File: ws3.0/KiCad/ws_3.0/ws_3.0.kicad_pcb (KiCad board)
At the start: 2 copper layers, 72.8 x 113.9 mm, 55 parts, among them J1 ISP TINY, J2 Rain, J3 Wind, J4 Temp, J5 2604-1102, J6 ISP MEGA, J7 FTDI MEGA, SW1 SW_DIP_x03, SW2 RESET TINY, SW3 RESET ATMEGA, U1 ATmega328P-A, U2 LF33_TO220, U3 ATtiny85V-10S, U4 XC6206PxxxMR, U5 RFM95W-868S2, Y1 Crystal

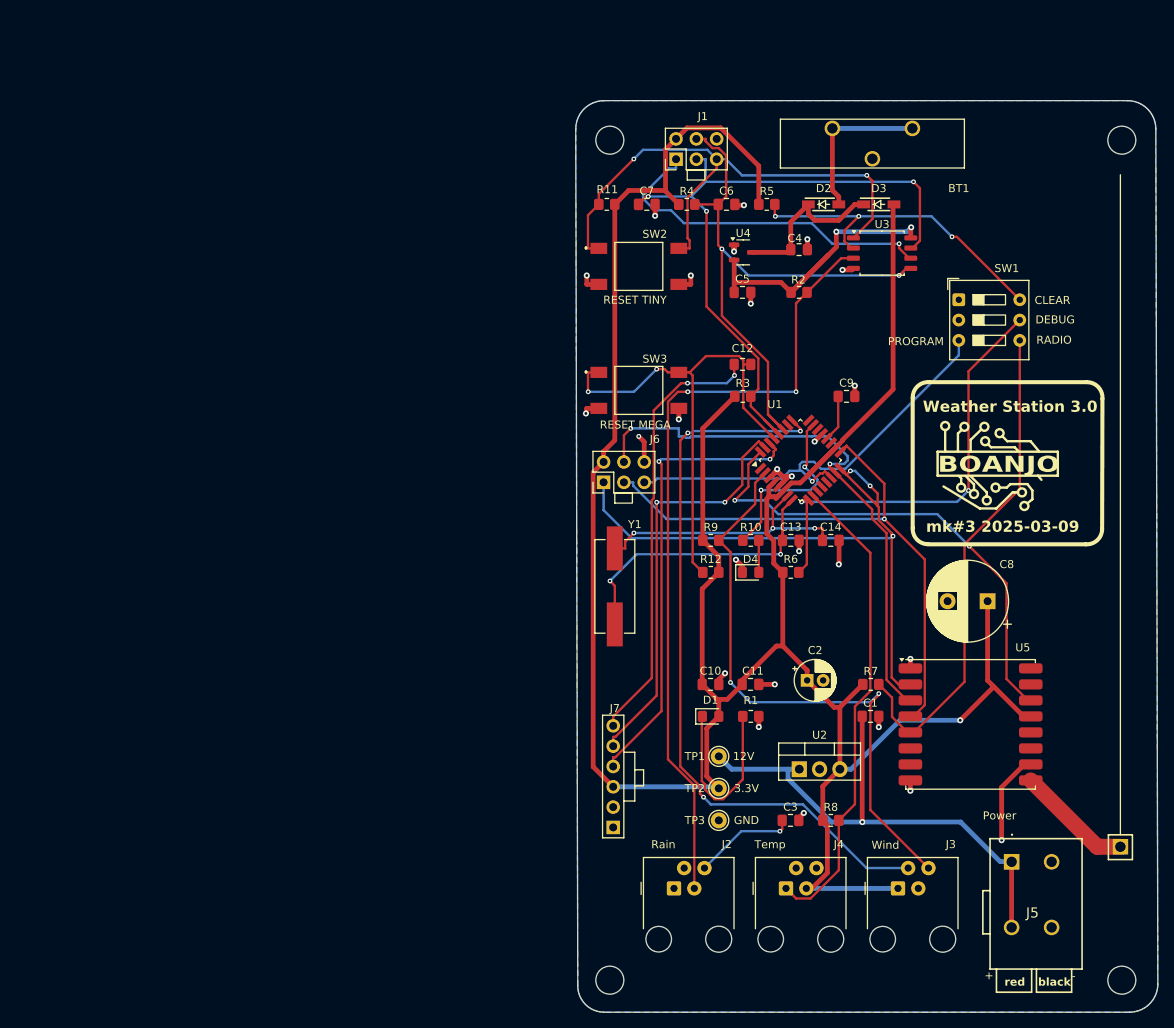
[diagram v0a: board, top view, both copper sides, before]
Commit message: Updates for mk #5
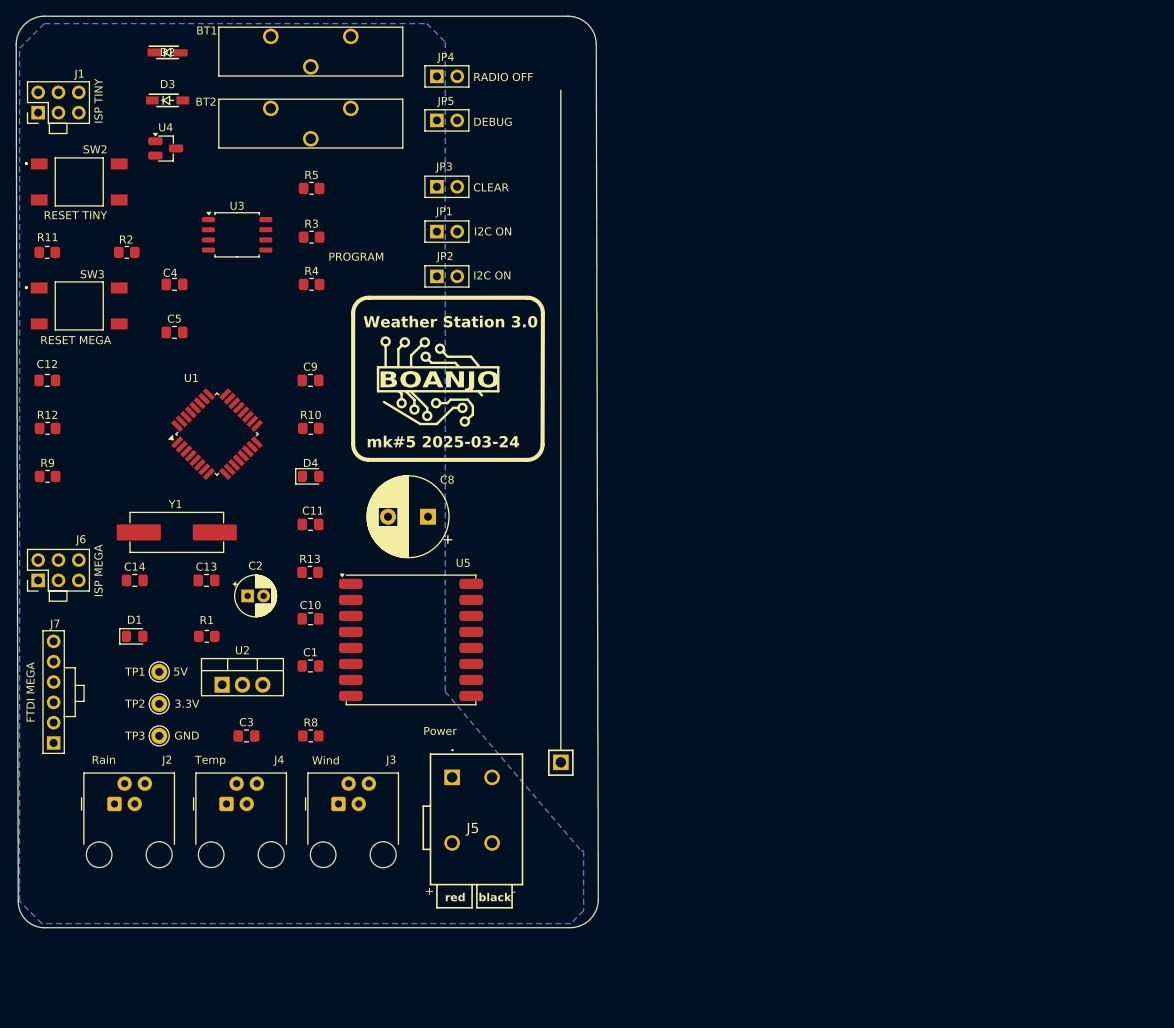
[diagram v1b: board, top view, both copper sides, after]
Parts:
- removed C6, C7: 0.1uF, Capacitor_SMD:C_0805_2012Metric_Pad1.18x1.45mm_HandSolder
- removed R6, R7: 4k7, Resistor_SMD:R_0805_2012Metric_Pad1.20x1.40mm_HandSolder
- removed SW1: SW_DIP_x03, Button_Switch_THT:SW_DIP_SPSTx03_Slide_9.78x9.8mm_W7.62mm_P2.54mm
- removed UNK_HOLE_0: , dummyfp0
- removed UNK_HOLE_1: , dummyfp1
- removed UNK_HOLE_2: , dummyfp2
- removed UNK_HOLE_3: , dummyfp3
- added BT2: CR2032, boan_devices:CR2032 standing 1074, F.Cu at (74.0, 49.0)
- added JP1: SCL, boan_devices:Jumper 2p, F.Cu at (96.1, 64.4)
- added JP2: SDA, boan_devices:Jumper 2p, F.Cu at (96.1, 70.0)
- added JP3: CLEAR, boan_devices:Jumper 2p, F.Cu at (96.1, 58.8)
- added JP4: PROGRAM MEGA, boan_devices:Jumper 2p, F.Cu at (96.1, 45.0)
- added JP5: DEBUG, boan_devices:Jumper 2p, F.Cu at (96.1, 50.5)
- added R13: 4k7, Resistor_SMD:R_0805_2012Metric_Pad1.20x1.40mm_HandSolder, F.Cu at (78.9, 107.0)
- D2: value 1N5819WS -> BAP70; footprint boan_devices:1N5819HW -> boan_devices:BAP70
- R1: value 330 -> 1k
- U4: footprint Package_TO_SOT_SMD:SOT-23-3 -> boan_devices:SOT-23
- moved D3 89.8 mm to (61.1, 48.0)
- moved C14 87.1 mm to (57.0, 108.0)
- moved C12 86.9 mm to (46.1, 83.0)
- moved R12 84.8 mm to (46.1, 89.0)
- moved R2 84.2 mm to (56.0, 67.0)
- moved D2 84.2 mm to (61.1, 42.0)
- moved R9 83.3 mm to (46.1, 95.0)
- moved U3 80.7 mm to (69.8, 64.8)
- moved J1 79.9 mm to (44.9, 49.5)
- moved C4 78.2 mm to (62.0, 71.0)
- moved U4 73.3 mm to (60.9, 54.0)
- moved C13 73.2 mm to (66.0, 108.0)
- moved U1 73.0 mm to (67.3, 89.7)
- moved U2 72.9 mm to (67.9, 121.0)
- moved D1 72.7 mm to (57.0, 115.0)
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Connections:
- BT1 pad 2: GND -> BAT
- C1 pad 1: /power/RAW -> RAW
- C12 pad 1: Net-(U1-~{RESET}/PC6) -> Net-(J6-~{RST})
- D3 pad 2: +3.3V -> RAW
- J1 pad 2: +3.3V -> RAW
- J1 pad 3: I2C_SCL -> Net-(J1-SCK)
- J1 pad 4: I2C_SDA -> Net-(J1-MOSI)
- J5 pad 1: /power/RAW -> RAW
- J5 pad 2: /power/RAW -> RAW
- J6 pad 2: +3.3V -> RAW
- J6 pad 5: SS -> Net-(J6-~{RST})
- R11 pad 2: +3.3V -> BACKUP_POWER
- R12 pad 1: Net-(U1-~{RESET}/PC6) -> Net-(J6-~{RST})
- R5 pad 1: +3.3V -> BACKUP_POWER
- SW3 pad 1: Net-(U1-~{RESET}/PC6) -> Net-(J6-~{RST})
- SW3 pad 3: Net-(U1-~{RESET}/PC6) -> Net-(J6-~{RST})
- TP1 pad 1: /power/RAW -> RAW
- U1 pad 14: SS -> NSS
- U1 pad 29: Net-(U1-~{RESET}/PC6) -> Net-(J6-~{RST})
- U2 pad 1: /power/RAW -> RAW
- U3 pad 5: I2C_SDA -> Net-(J1-MOSI)
- U3 pad 7: I2C_SCL -> Net-(J1-SCK)
- U5 pad 5: OPT_PROGRAM -> NSS
- U5 pad 6: unconnected-(U5-RESET-Pad6) -> Net-(U5-RESET)
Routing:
- net +3.3V: track 353.4 -> 0.00 mm, vias 1 -> 0
- net RAIN: track 99.3 -> 0.00 mm, vias 2 -> 0
- net WIND_DIR: track 93.0 -> 0.00 mm, vias 3 -> 0
- net I2C_SCL: track 86.9 -> 0.00 mm, vias 3 -> 0
- net MISO: track 80.8 -> 0.00 mm, vias 3 -> 0
- net SCK: track 75.7 -> 0.00 mm, vias 1 -> 0
- net WIND_SPEED: track 75.0 -> 0.00 mm, vias 2 -> 0
- net I2C_SDA: track 73.7 -> 0.00 mm, vias 2 -> 0
- net MOSI: track 71.9 -> 0.00 mm, vias 2 -> 0
- net Net-(J1-~{RST}): track 69.0 -> 0.00 mm, vias 2 -> 0
- net /power/RAW: track 65.6 -> 0.00 mm, vias 1 -> 0
- net Net-(U1-~{RESET}/PC6): track 63.6 -> 0.00 mm, vias 2 -> 0
- net OPT_PROGRAM: track 62.8 -> 0.00 mm
- net DIO0: track 61.7 -> 0.00 mm, vias 2 -> 0
- net GND: track 61.3 -> 0.00 mm, vias 26 -> 0
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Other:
- board text added: "5V"
- board text added: "FTDI MEGA"
- board text added: "I2C ON"
- board text added: "RADIO OFF"
- board text added: "mk#5 2025-03-24"
- board text removed: "12V"
- board text removed: "RADIO"
- board text removed: "mk#3 2025-03-09"

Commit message: PCBWAYs delivery 2025-04-16 mk#5 of ws3.0
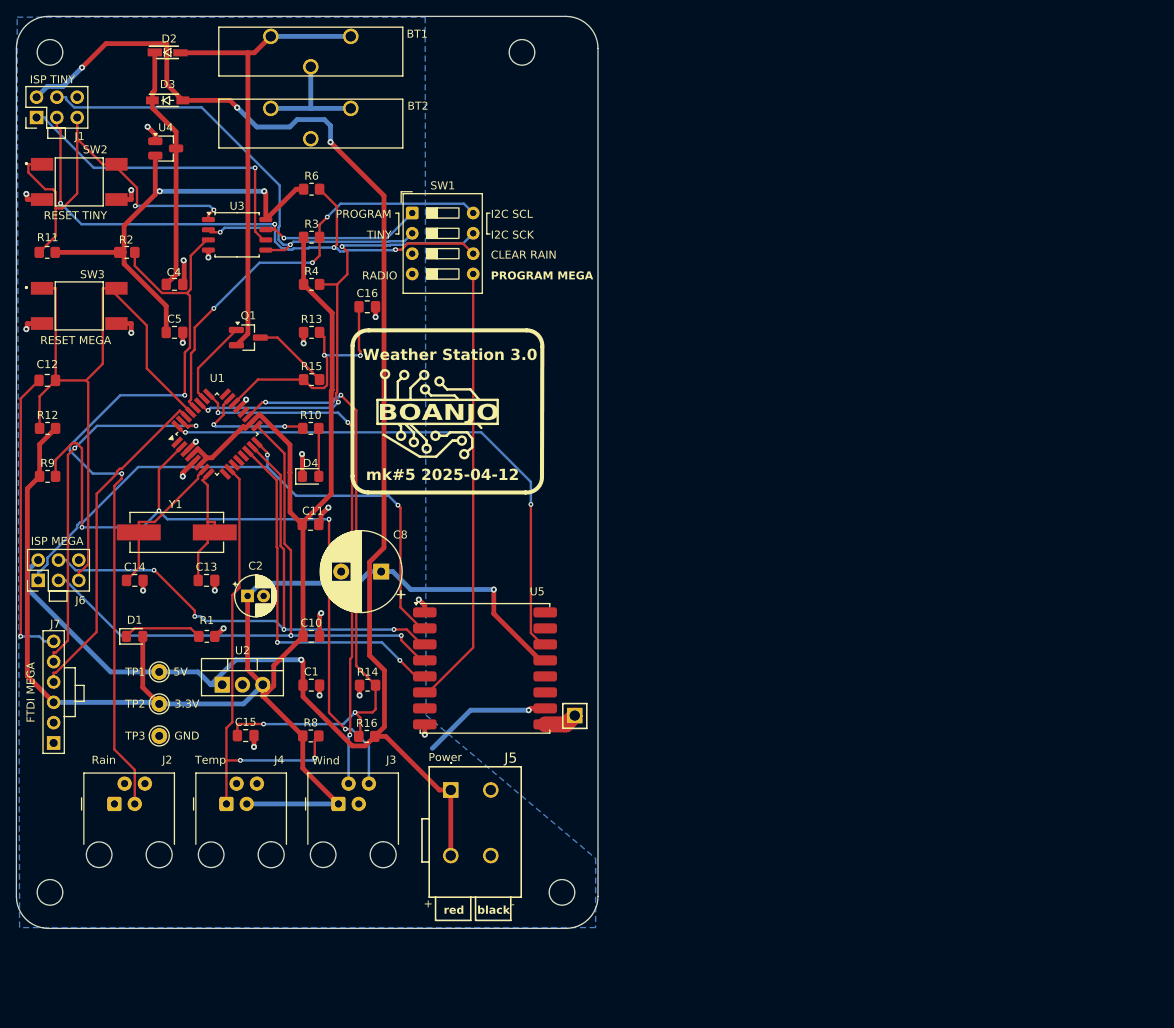
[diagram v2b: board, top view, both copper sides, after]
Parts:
- removed C3, C9: 0.1uF, Capacitor_SMD:C_0805_2012Metric_Pad1.18x1.45mm_HandSolder
- removed JP1: SCL, boan_devices:Jumper 2p
- removed JP2: SDA, boan_devices:Jumper 2p
- removed JP3: CLEAR, boan_devices:Jumper 2p
- removed JP4: PROGRAM MEGA, boan_devices:Jumper 2p
- removed JP5: DEBUG, boan_devices:Jumper 2p
- removed R5: 4k7, Resistor_SMD:R_0805_2012Metric_Pad1.20x1.40mm_HandSolder
- added C15: 0.1uF, Capacitor_SMD:C_0805_2012Metric_Pad1.18x1.45mm_HandSolder, F.Cu at (70.9, 127.4)
- added C16: 0.1uF, Capacitor_SMD:C_0805_2012Metric_Pad1.18x1.45mm_HandSolder, F.Cu at (86.1, 73.8)
- added MH1: MountingHole_3.2mm_M3, MountingHole:MountingHole_3.2mm_M3, F.Cu at (46.4, 42.0)
- added MH2: MountingHole_3.2mm_M3, MountingHole:MountingHole_3.2mm_M3, F.Cu at (105.4, 42.0)
- added MH3: MountingHole_3.2mm_M3, MountingHole:MountingHole_3.2mm_M3, F.Cu at (46.4, 147.0)
- added MH4: MountingHole_3.2mm_M3, MountingHole:MountingHole_3.2mm_M3, F.Cu at (110.4, 147.0)
- added Q1: ISS55EP06LMXTSA1, Package_TO_SOT_SMD:SOT-23_Handsoldering, F.Cu at (71.2, 77.7)
- added R14: 100k, Resistor_SMD:R_0805_2012Metric_Pad1.20x1.40mm_HandSolder, F.Cu at (86.1, 121.1)
- added R15: 560k, Resistor_SMD:R_0805_2012Metric_Pad1.20x1.40mm_HandSolder, F.Cu at (79.1, 82.9)
- added R16: 560k, Resistor_SMD:R_0805_2012Metric_Pad1.20x1.40mm_HandSolder, F.Cu at (86.0, 127.5)
- added R6: 4k7, Resistor_SMD:R_0805_2012Metric_Pad1.20x1.40mm_HandSolder, F.Cu at (79.1, 59.1)
- added SW1: SW_DIP_x04, Button_Switch_THT:SW_DIP_SPSTx04_Slide_9.78x12.34mm_W7.62mm_P2.54mm, F.Cu at (91.7, 62.1)
- R13: value 4k7 -> 100k
- moved R13 30.0 mm to (79.1, 77.0)
- moved U5 9.90 mm to (100.8, 119.0)
- moved C8 9.02 mm to (87.8, 106.9)
- moved AE1 6.10 mm to (112.0, 125.0)
- moved C1 2.40 mm to (79.1, 121.1)
- moved C10 2.20 mm to (79.1, 115.0)
- moved J5 1.58 mm to (96.5, 134.2)
- moved J1 0.63 mm to (44.7, 50.1)
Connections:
- net /Attiny85/BATTERY renamed BACKUP_BATTERY
- J2 pad 4: Net-(C3-Pad1) -> GND
- R13 pad 1: +3.3V -> GND
- R13 pad 2: OPT_DEBUG -> Net-(U1-ADC7)
- U1 pad 19: unconnected-(U1-ADC6-Pad19) -> Net-(U1-ADC6)
- U1 pad 20: Net-(U1-AREF) -> unconnected-(U1-AREF-Pad20)
- U1 pad 22: unconnected-(U1-ADC7-Pad22) -> Net-(U1-ADC7)
- U1 pad 26: unconnected-(U1-PC3-Pad26) -> BACKUP_DIV_CTRL
- U1 pad 9: OPT_DEBUG -> unconnected-(U1-PD5-Pad9)
- U5 pad 6: Net-(U5-RESET) -> DISABLE_RADIO
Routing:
- net +3.3V: track 0.00 -> 252.3 mm, vias 0 -> 1
- net RAW: track 0.00 -> 211.8 mm, vias 0 -> 4
- net RAIN: track 0.00 -> 98.7 mm, vias 0 -> 2
- net WIND_SPEED: track 0.00 -> 93.3 mm, vias 0 -> 4
- net Net-(J6-~{RST}): track 0.00 -> 83.4 mm
- net SCK: track 0.00 -> 78.4 mm, vias 0 -> 2
- net Net-(U1-ADC6): track 0.00 -> 76.8 mm, vias 0 -> 4
- net MOSI: track 0.00 -> 75.2 mm, vias 0 -> 4
- net MISO: track 0.00 -> 74.8 mm, vias 0 -> 2
- net DIO0: track 0.00 -> 68.4 mm, vias 0 -> 2
- net WIND_DIR: track 0.00 -> 65.1 mm, vias 0 -> 3
- net GND: track 0.00 -> 63.1 mm, vias 0 -> 25
- net Net-(J1-MOSI): track 0.00 -> 60.3 mm, vias 0 -> 1
- net Net-(J1-SCK): track 0.00 -> 59.5 mm, vias 0 -> 3
- net BACKUP_BATTERY: track 0.00 -> 59.3 mm
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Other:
- board size 72.8 x 113.9 mm -> 72.7 x 114 mm
- board text added: "CLEAR RAIN"
- board text added: "I2C SCK"
- board text added: "I2C SCL"
- board text added: "PROGRAM MEGA"
- board text added: "RADIO"
- board text added: "TINY"
- board text added: "mk#5 2025-04-12"
- board text removed: "CLEAR"
- board text removed: "DEBUG"
- board text removed: "I2C ON"
- board text removed: "RADIO OFF"
- board text removed: "mk#5 2025-03-24"
